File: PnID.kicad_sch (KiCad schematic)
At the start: 14 parts

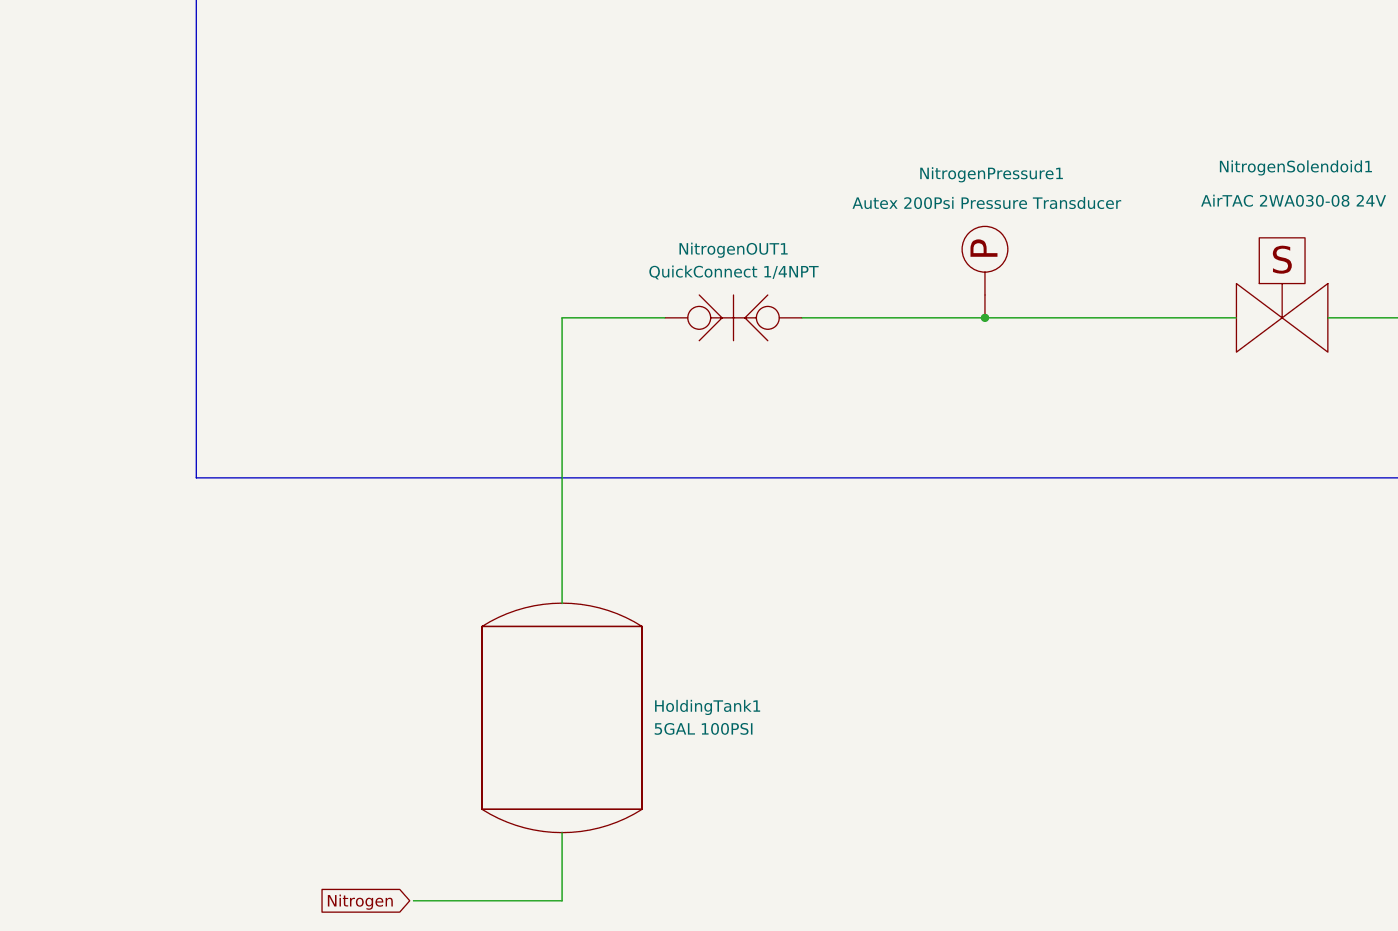
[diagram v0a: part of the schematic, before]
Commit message: .
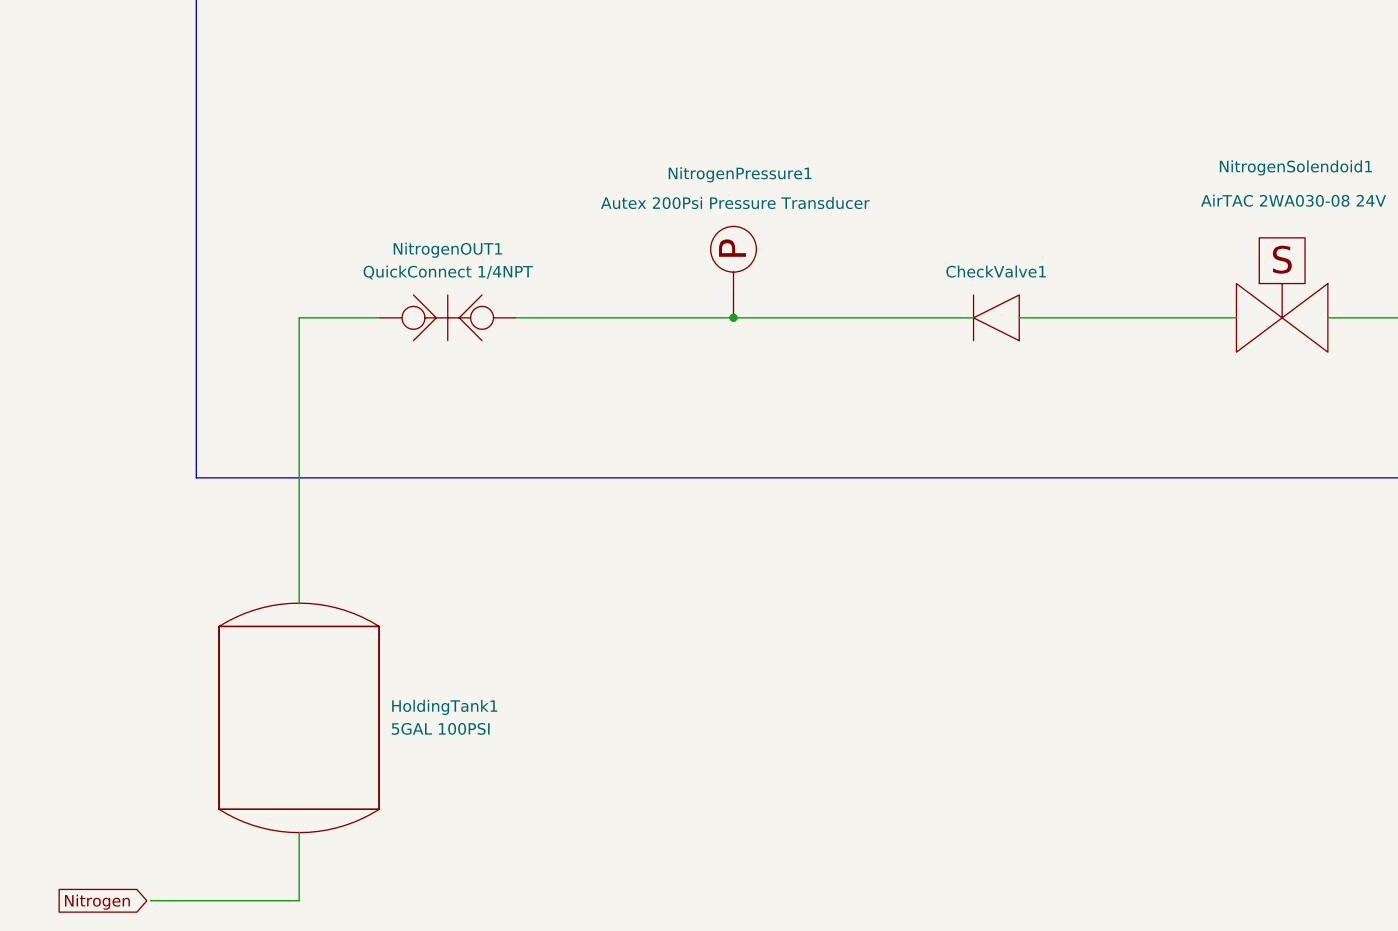
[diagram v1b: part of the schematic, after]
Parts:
- added CheckValve1: CheckValve, symbol pnid-lib:CheckValve
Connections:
- net at NitrogenMembrane1.~: now also AirOUT1.~; no longer NitrogenIN1.~
- net at AirOUT1.~: now also AirNeedleValve1.~; no longer NitrogenMembrane1.~
- net at HoldingTank1.~: now also NitrogenOUT1.~
- net at NitrogenOUT1.~: now also NitrogenPressure1.~, CheckValve1.~; no longer HoldingTank1.~
- net at NitrogrenNeedleValve1.~: now also NitrogenIN1.~; no longer NitrogenSolendoid1.~
- net at AirIN1.~: no longer Compressor1.~
- new net: NitrogenIN1.~, NitrogenMembrane1.~
- new net: AirNeedleValve1.~, AirPressure1.~, AirSolenoid1.~
- new net: NitrogenSolendoid1.~, NitrogrenNeedleValve1.~
- new net: CheckValve1.~, NitrogenSolendoid1.~
- new net: AirIN1.~, Compressor1.~
- now unconnected: AirSolenoid1.~
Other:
- moved on the sheet: HoldingTank1, NitrogenOUT1, NitrogenPressure1
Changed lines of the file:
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@@
 	)
 	(junction
-		(at 129.54 116.84)
+		(at 101.6 116.84)
 		(diameter 0)
 		(color 0 0 0 0)
@@
 	(wire
 		(pts
-			(xy 109.22 116.84) (xy 129.54 116.84)
+			(xy 77.47 116.84) (xy 101.6 116.84)
 		)
 		(stroke
@@
 	(wire
 		(pts
-			(xy 82.55 116.84) (xy 93.98 116.84)
+			(xy 53.34 116.84) (xy 62.23 116.84)
 		)
 		(stroke
@@
 	(wire
 		(pts
-			(xy 66.04 181.61) (xy 82.55 181.61)
+			(xy 36.83 181.61) (xy 53.34 181.61)
+		)
+		(stroke
+			(width 0)
+			(type default)
+		)
+	)
+	(wire
+		(pts
+			(xy 133.35 116.84) (xy 157.48 116.84)
+		)
+		(stroke
+			(width 0)
+			(type default)
+		)
+	)
+	(wire
+		(pts
+			(xy 101.6 116.84) (xy 128.27 116.84)
 		)
 		(stroke
@@
 	(wire
 		(pts
-			(xy 82.55 173.99) (xy 82.55 181.61)
+			(xy 53.34 173.99) (xy 53.34 181.61)
 		)
 		(stroke
@@
 	(wire
 		(pts
-			(xy 82.55 116.84) (xy 82.55 148.59)
+			(xy 53.34 116.84) (xy 53.34 148.59)
 		)
 		(stroke
@@
 			(type dash)
 			(color 132 0 0 1)
-		)
-	)
-	(wire
-		(pts
-			(xy 129.54 116.84) (xy 157.48 116.84)
-		)
-		(stroke
-			(width 0)
-			(type default)
 		)
 	)
@@
 	(global_label "Nitrogen"
 		(shape output)
-		(at 55.88 181.61 0)
+		(at 26.67 181.61 0)
 		(fields_autoplaced yes)
 		(effects
@@
 		)
 		(property "Intersheetrefs" "${INTERSHEET_REFS}"
-			(at 66.848 181.61 0)
+			(at 37.638 181.61 0)
 			(effects
 				(font
@@
 	(symbol
 		(lib_id "pnid-lib:Tank")
-		(at 82.55 161.29 0)
+		(at 53.34 161.29 0)
 		(unit 1)
 		(exclude_from_sim no)
@@
 		(fields_autoplaced yes)
 		(property "Reference" "HoldingTank1"
-			(at 92.71 160.0199 0)
+			(at 63.5 160.0199 0)
 			(effects
 				(font
@@
 		)
 		(property "Value" "5GAL 100PSI"
-			(at 92.71 162.5599 0)
+			(at 63.5 162.5599 0)
 			(effects
 				(font
@@
 		)
 		(property "Footprint" ""
-			(at 82.55 161.29 0)
+			(at 53.34 161.29 0)
 			(effects
 				(font
@@
 		)
 		(property "Datasheet" ""
-			(at 82.55 161.29 0)
+			(at 53.34 161.29 0)
 			(effects
 				(font
@@
 		)
 		(property "Description" ""
-			(at 82.55 161.29 0)
+			(at 53.34 161.29 0)
 			(effects
 				(font
@@
 		)
 		(property "Unit" "%"
-			(at 82.55 161.29 0)
+			(at 53.34 161.29 0)
 			(effects
 				(font
@@
 		)
 		(property "Action_Reference" " "
-			(at 82.55 161.29 0)
+			(at 53.34 161.29 0)
 			(effects
 				(font
@@
 		)
 		(property "Data_Content" " "
-			(at 82.55 161.29 0)
+			(at 53.34 161.29 0)
 			(effects
 				(font
@@
 	)
 	(symbol
+		(lib_id "pnid-lib:CheckValve")
+		(at 130.81 116.84 180)
+		(unit 1)
+		(exclude_from_sim no)
+		(in_bom yes)
+		(on_board yes)
+		(dnp no)
+		(fields_autoplaced yes)
+		(property "Reference" "CheckValve1"
+			(at 130.81 111.76 0)
+			(effects
+				(font
+					(size 1.27 1.27)
+				)
+			)
+		)
+		(property "Value" "CheckValve"
+			(at 130.81 112.522 0)
+			(effects
+				(font
+					(size 0.508 0.508)
+				)
+				(hide yes)
+			)
+		)
+		(property "Footprint" ""
+			(at 130.81 116.84 0)
+			(effects
+				(font
+					(size 0.508 0.508)
+				)
+				(hide yes)
+			)
+		)
+		(property "Datasheet" ""
+			(at 130.81 116.84 0)
+			(effects
+				(font
+					(size 0.508 0.508)
+				)
+				(hide yes)
+			)
+		)
+		(property "Description" ""
+			(at 130.81 116.84 0)
+			(effects
+				(font
+					(size 1.27 1.27)
+				)
+				(hide yes)
+			)
+		)
+		(pin "~"
+		)
+		(pin "~"
+		)
+		(instances
+			(project ""
+				(path "/c5365556-9b4a-4e37-8bb8-20fd18113201/1b754a42-13ad-4d8b-8663-062e1b8a93f8"
+					(reference "CheckValve1")
+					(unit 1)
+				)
+			)
+		)
+	)
+	(symbol
 		(lib_id "pnid-lib:Valve_Needle")
 		(at 196.85 69.85 0)
@@
 	(symbol
 		(lib_id "pnid-lib:Sensor_Pressure")
-		(at 129.54 109.22 90)
+		(at 101.6 109.22 90)
 		(unit 1)
 		(exclude_from_sim no)
@@
 		(dnp no)
 		(property "Reference" "NitrogenPressure1"
-			(at 122.174 100.838 90)
+			(at 94.234 100.838 90)
 			(effects
 				(font
@@
 		)
 		(property "Value" "Autex 200Psi Pressure Transducer"
-			(at 114.808 104.14 90)
+			(at 86.868 104.14 90)
 			(effects
 				(font
@@
 		)
 		(property "Footprint" ""
-			(at 129.54 109.22 0)
+			(at 101.6 109.22 0)
 			(effects
 				(font
@@
 		)
 		(property "Datasheet" ""
-			(at 129.54 109.22 0)
+			(at 101.6 109.22 0)
 			(effects
 				(font
@@
 		)
 		(property "Description" ""
-			(at 129.54 109.22 0)
+			(at 101.6 109.22 0)
 			(effects
 				(font
@@
 		)
 		(property "Unit" "bar"
-			(at 129.54 109.22 0)
+			(at 101.6 109.22 0)
 			(effects
 				(font
@@
 		)
 		(property "Action_Reference" " "
-			(at 129.54 109.22 0)
+			(at 101.6 109.22 0)
 			(effects
 				(font
@@
 		)
 		(property "Data_Content" " "
-			(at 133.35 113.0299 90)
+			(at 105.41 113.0299 90)
 			(effects
 				(font
@@
 		(lib_name "QuickConnect_1")
 		(lib_id "pnid-lib:QuickConnect")
-		(at 101.6 116.84 0)
+		(at 69.85 116.84 0)
 		(unit 1)
 		(exclude_from_sim no)
@@
 		(fields_autoplaced yes)
 		(property "Reference" "NitrogenOUT1"
-			(at 101.6 109.22 0)
+			(at 69.85 109.22 0)
 			(effects
 				(font
@@
 		)
 		(property "Value" "QuickConnect 1/4NPT"
-			(at 101.6 111.76 0)
+			(at 69.85 111.76 0)
 			(effects
 				(font
@@
 		)
 		(property "Footprint" ""
-			(at 101.6 116.84 0)
+			(at 69.85 116.84 0)
 			(effects
 				(font
@@
 		)
 		(property "Datasheet" ""
-			(at 101.6 116.84 0)
+			(at 69.85 116.84 0)
 			(effects
 				(font
@@
 		)
 		(property "Description" ""
-			(at 101.6 116.84 0)
-			(effects
-				(font
+			(at 69.85 116.84 0)
+			(effects
+				(font
